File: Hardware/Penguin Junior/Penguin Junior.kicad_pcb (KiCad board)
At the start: 4 copper layers, 58.5 x 25.4 mm, 117 parts, among them J1 Conn_02x05_SWD, J10 Conn_01x10, J11 Conn_01x10, J12 Conn_01x06_UART, J13 Conn_01x04_UART, J14 Conn_01x01, J2 Conn_02x05_SWD, J3 Micro_SD_Card_Det1, J4 Conn_01x03_Video, J5 USB_B_Micro, J6 Conn_01x03_Video, J7 Conn_01x06_UART, J8 Conn_01x04_I2C, J9 Conn_01x10, Q1 BSS138, SW1 SW_Push, U1 STM32F405RGTx, U2 MS5611-01BA, U3 BMI088, U4 MAX7456, U5 ST1S14PHR, U6 INA219AxD, U7 LDL1117_3V3, Y1 16MHz, Y2 27MHz

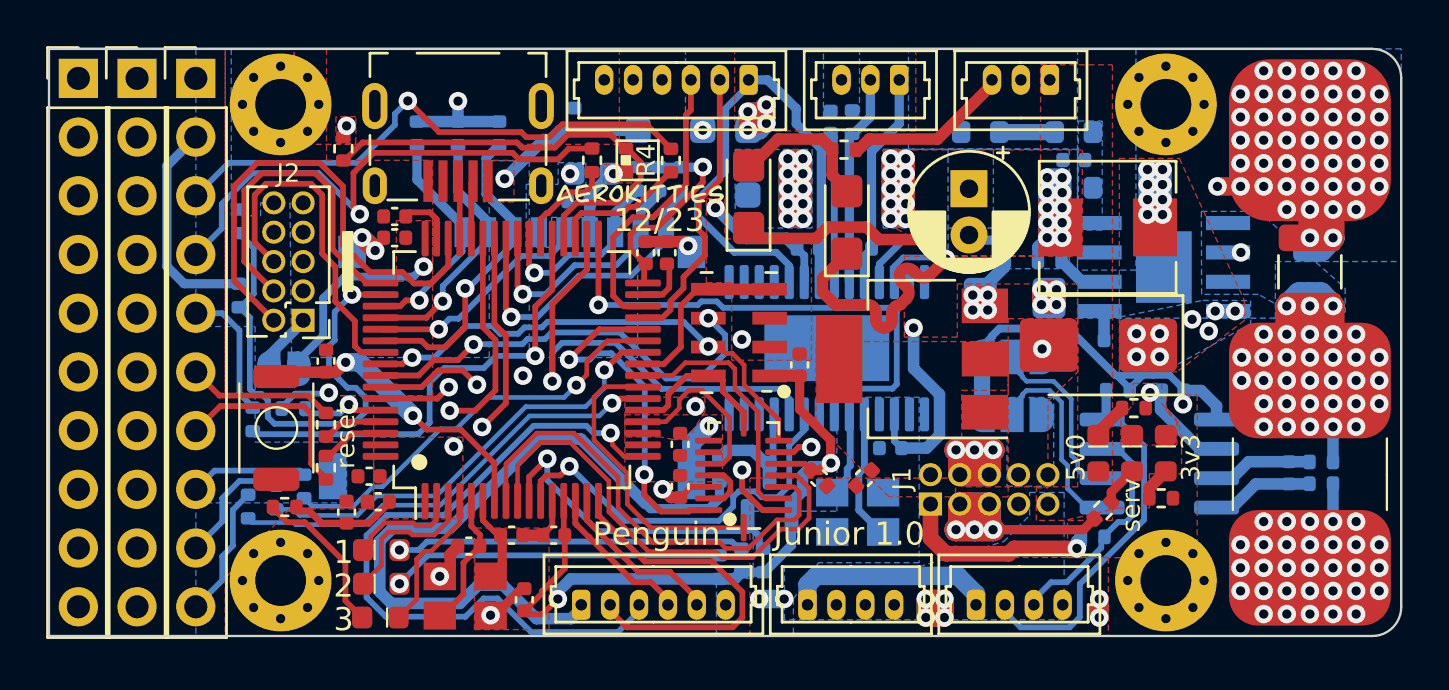
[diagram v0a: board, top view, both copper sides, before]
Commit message: Updated Penguin project
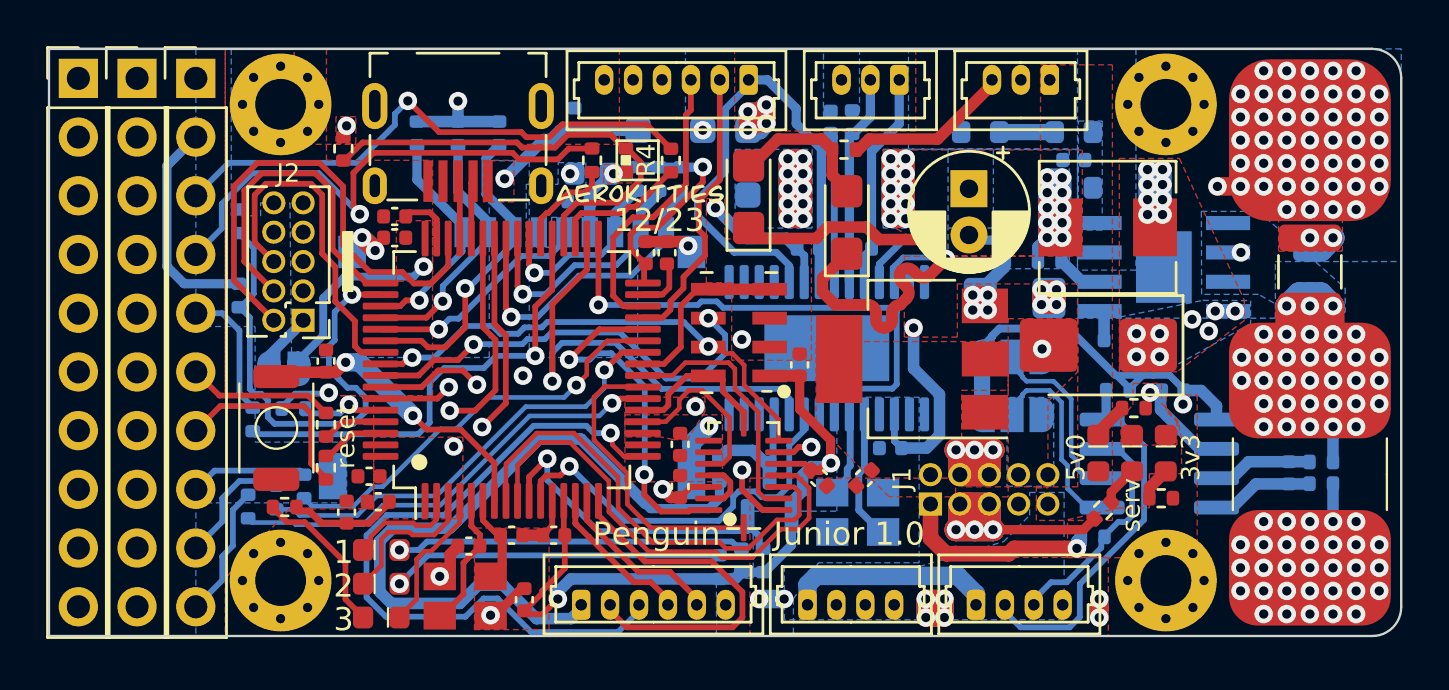
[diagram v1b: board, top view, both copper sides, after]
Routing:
- net GND: track 90.7 -> 88.2 mm
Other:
- board text added: "25.4x58.5"
- board text removed: "locked"
- board text removed: "ПРОВЕРИТЬ ТАЙМЕРЫ!!!"

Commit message: Updated Penguin project
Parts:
- R17, R18, R19, R22, R23, R24, R25, R26, R27, R28, R30, R31: value 22 -> 220
- R4, R5: value 33 -> 330
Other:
- board text added: "РЕЗИСТОРЫ НА ЗАБОРЕ 22 -> 220 зачем они вообще и чем плохи большие (плюсы -- универсальность)"
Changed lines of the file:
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@@
         (effects (font (size 0.8 0.8) (thickness 0.12)))
     )
-    (fp_text value "33" (at 0 1.17 90) (layer "F.Fab")
+    (fp_text value "330" (at 0 1.17 90) (layer "F.Fab")
         (effects (font (size 1 1) (thickness 0.15)))
     )
@@
         (effects (font (size 1 1) (thickness 0.15)))
     )
-    (fp_text value "22" (at 0 1.17 90) (layer "F.Fab")
+    (fp_text value "220" (at 0 1.17 90) (layer "F.Fab")
         (effects (font (size 1 1) (thickness 0.15)))
     )
@@
         (effects (font (size 1 1) (thickness 0.15)))
     )
-    (fp_text value "22" (at 0 1.17 90) (layer "F.Fab")
+    (fp_text value "220" (at 0 1.17 90) (layer "F.Fab")
         (effects (font (size 1 1) (thickness 0.15)))
     )
@@
         (effects (font (size 1 1) (thickness 0.15)))
     )
-    (fp_text value "22" (at 0 1.17 90) (layer "F.Fab")
+    (fp_text value "220" (at 0 1.17 90) (layer "F.Fab")
         (effects (font (size 1 1) (thickness 0.15)))
     )
@@
         (effects (font (size 1 1) (thickness 0.15)))
     )
-    (fp_text value "22" (at 0 1.17 90) (layer "F.Fab")
+    (fp_text value "220" (at 0 1.17 90) (layer "F.Fab")
         (effects (font (size 1 1) (thickness 0.15)))
     )
@@
         (effects (font (size 1 1) (thickness 0.15)))
     )
-    (fp_text value "22" (at 0 1.17 90) (layer "F.Fab")
+    (fp_text value "220" (at 0 1.17 90) (layer "F.Fab")
         (effects (font (size 1 1) (thickness 0.15)))
     )
@@
         (effects (font (size 1 1) (thickness 0.15)) (justify mirror))
     )
-    (fp_text value "22" (at 0 -1.17 90) (layer "B.Fab")
+    (fp_text value "220" (at 0 -1.17 90) (layer "B.Fab")
         (effects (font (size 1 1) (thickness 0.15)) (justify mirror))
     )
@@
         (effects (font (size 1 1) (thickness 0.15)) (justify mirror))
     )
-    (fp_text value "22" (at 0 -1.17 270) (layer "B.Fab")
+    (fp_text value "220" (at 0 -1.17 270) (layer "B.Fab")
         (effects (font (size 1 1) (thickness 0.15)) (justify mirror))
     )
@@
         (effects (font (size 0.8 0.8) (thickness 0.12)) (justify mirror))
     )
-    (fp_text value "33" (at 0 -1.17 -90) (layer "B.Fab")
+    (fp_text value "330" (at 0 -1.17 -90) (layer "B.Fab")
         (effects (font (size 1 1) (thickness 0.15)) (justify mirror))
     )
@@
         (effects (font (size 1 1) (thickness 0.15)) (justify mirror))
     )
-    (fp_text value "22" (at 0 -1.17 90) (layer "B.Fab")
+    (fp_text value "220" (at 0 -1.17 90) (layer "B.Fab")
         (effects (font (size 1 1) (thickness 0.15)) (justify mirror))
     )
@@
         (effects (font (size 1 1) (thickness 0.15)) (justify mirror))
     )
-    (fp_text value "22" (at 0 -1.17) (layer "B.Fab")
+    (fp_text value "220" (at 0 -1.17) (layer "B.Fab")
         (effects (font (size 1 1) (thickness 0.15)) (justify mirror))
     )
@@
         (effects (font (size 1 1) (thickness 0.15)) (justify mirror))
     )
-    (fp_text value "22" (at 0 -1.17) (layer "B.Fab")
+    (fp_text value "220" (at 0 -1.17) (layer "B.Fab")
         (effects (font (size 1 1) (thickness 0.15)) (justify mirror))
     )
@@
         (effects (font (size 1 1) (thickness 0.15)) (justify mirror))
     )
-    (fp_text value "22" (at 0 -1.17 90) (layer "B.Fab")
+    (fp_text value "220" (at 0 -1.17 90) (layer "B.Fab")
         (effects (font (size 1 1) (thickness 0.15)) (justify mirror))
     )
@@
         (effects (font (size 1 1) (thickness 0.15)) (justify mirror))
     )
-    (fp_text value "22" (at 0 -1.17 -90) (layer "B.Fab")
+    (fp_text value "220" (at 0 -1.17 -90) (layer "B.Fab")
         (effects (font (size 1 1) (thickness 0.15)) (justify mirror))
     )
@@
     )
   )
+  (gr_text "РЕЗИСТОРЫ НА ЗАБОРЕ 22 -> 220\n\nзачем они вообще и чем плохи большие\n\n(плюсы -- универсальность)" (at 115.82 100.24) (layer "User.2")
+    (effects (font (size 1 1) (thickness 0.15)) (justify left bottom))
+  )
   (gr_text "25.4x58.5\n" (at 92.755 60.74) (layer "User.2")
